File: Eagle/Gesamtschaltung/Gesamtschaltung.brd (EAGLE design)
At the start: 102.2 x 83.5 mm, 83 parts, among them IC03 LP2950CDT-3.3, IC1 MC9S08AW60, Q1 4M9152, Q2 P5N50

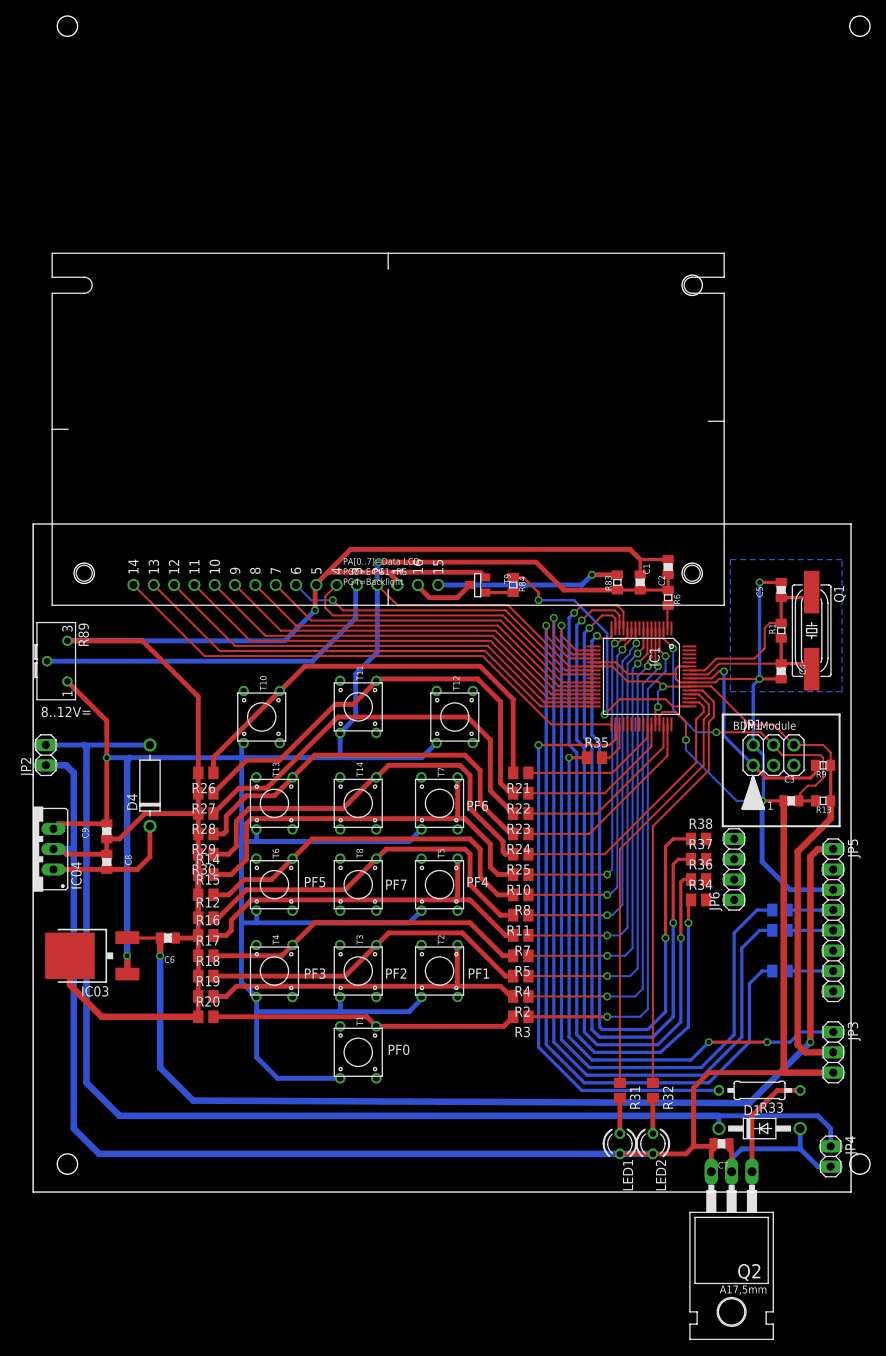
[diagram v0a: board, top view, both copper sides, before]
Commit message: edit Dokumentation, add diverse Bilder
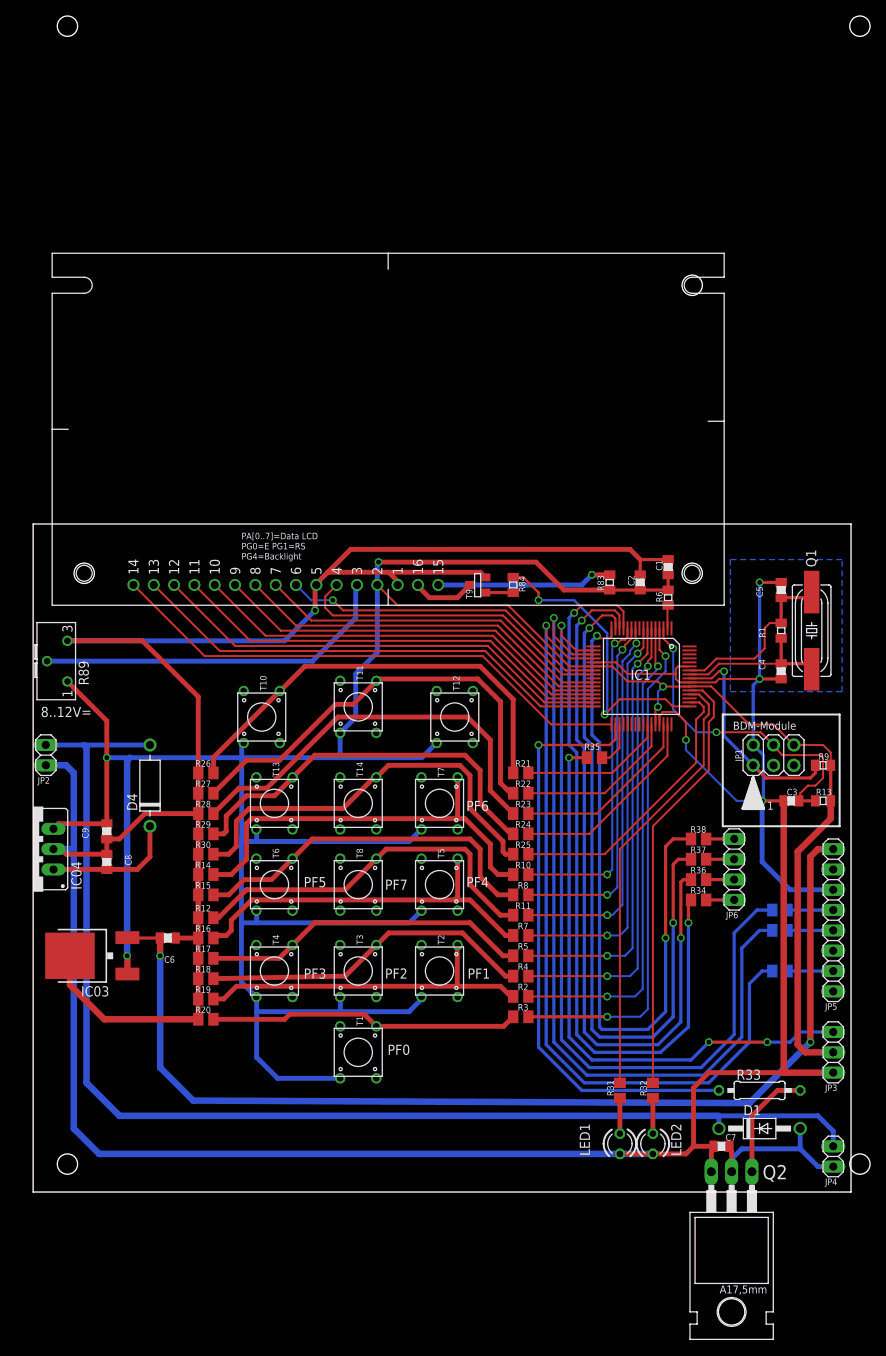
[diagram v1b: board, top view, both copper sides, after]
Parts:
- LED1: value (none) -> RED
- LED2: value (none) -> GREEN
- moved R83 0.95 mm to (72.7, 76.5)
- moved R20 0.32 mm to (22.2, 21.9)
- moved C7 0.32 mm to (86.7, 6.03)
- moved R17 0.32 mm to (22.2, 29.5)
- moved R18 0.32 mm to (22.2, 27.0)
- moved R19 0.32 mm to (22.2, 24.4)
- moved JP4 0.32 mm to (100.6, 4.76)
- moved R16 0.32 mm to (22.2, 32.1)
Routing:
- net N$57: track 0.00 -> 3.50 mm
- net N$56: track 0.00 -> 3.50 mm
- net N$54: track 0.00 -> 3.50 mm
- net N$45: track 0.00 -> 3.50 mm
- net N$86: track 22.9 -> 22.0 mm
